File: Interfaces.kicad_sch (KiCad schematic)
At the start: 15 parts, among them J1 I/O_HDR, J2 UART1_HDR, J7 I2C2_Headers, J9 I2C1_Headers

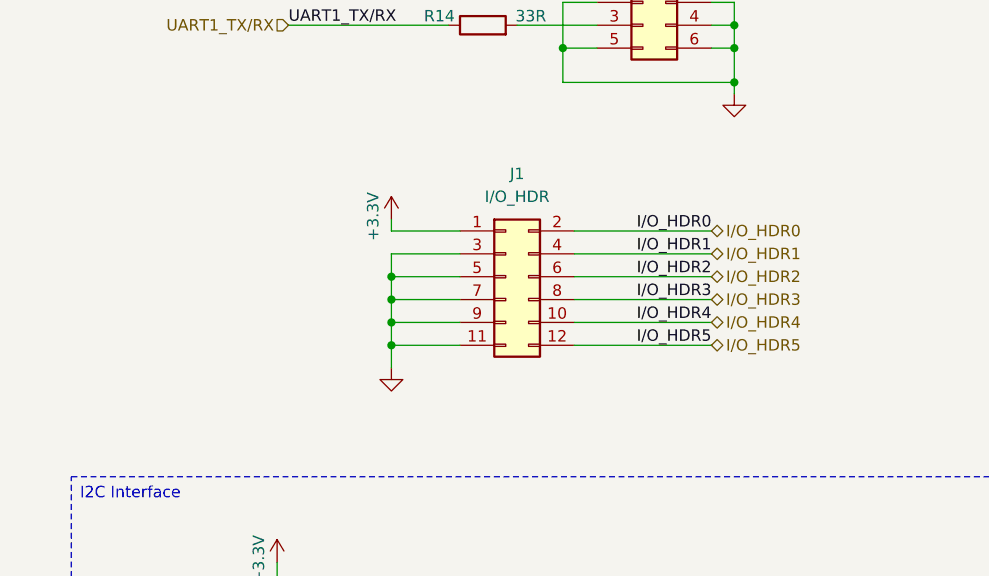
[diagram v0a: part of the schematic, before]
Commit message: Power domain update
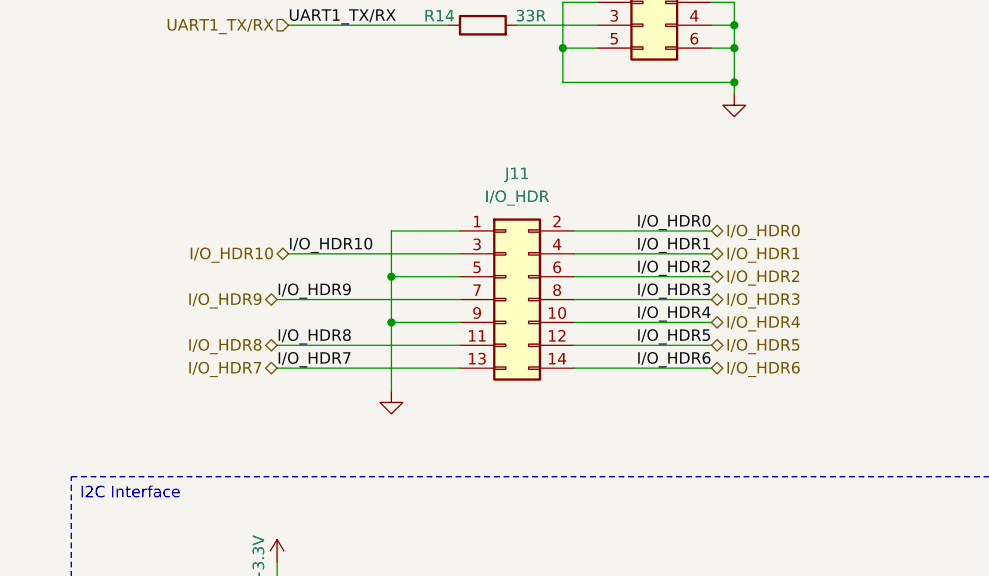
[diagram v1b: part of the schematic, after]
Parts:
- removed J1: I/O_HDR, Connector_PinHeader_2.54mm:PinHeader_2x06_P2.54mm_Horizontal, symbol Connector_Generic:Conn_02x06_Odd_Even
- added J11: I/O_HDR, Connector_PinHeader_2.54mm:PinHeader_2x07_P2.54mm_Horizontal, symbol Connector_Generic:Conn_02x07_Odd_Even
- J2, J9: footprint Connector_PinHeader_2.54mm:PinHeader_2x03_P2.54mm_Horizontal -> Personal_Projects:PinHeader_2x03_P2.54mm_Horizontal_Court
- J7: footprint Connector_PinHeader_2.54mm:PinHeader_2x03_P2.54mm_Horizontal -> Personal_Project:PinHeader_2x03_P2.54mm_Horizontal_Court
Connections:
- net GND: now also J11.1 (Pin_1), J11.5 (Pin_5), J11.9 (Pin_9)
- net I/O_HDR0: now also J11.2 (Pin_2)
- net I/O_HDR1: now also J11.4 (Pin_4)
- net I/O_HDR2: now also J11.6 (Pin_6)
- net I/O_HDR3: now also J11.8 (Pin_8)
- net I/O_HDR4: now also J11.10 (Pin_10)
- net I/O_HDR5: now also J11.12 (Pin_12)
- new net I/O_HDR10: J11.3 (Pin_3)
- new net I/O_HDR6: J11.14 (Pin_14)
- new net I/O_HDR7: J11.13 (Pin_13)
- new net I/O_HDR8: J11.11 (Pin_11)
- new net I/O_HDR9: J11.7 (Pin_7)
